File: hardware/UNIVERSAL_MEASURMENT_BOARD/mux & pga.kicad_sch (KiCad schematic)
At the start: 11 parts, among them U3 PGA280AIPW, U4 CD4097BM

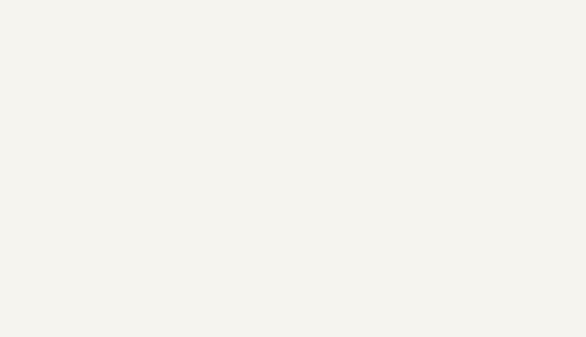
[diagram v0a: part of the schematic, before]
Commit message: clean up project visuals
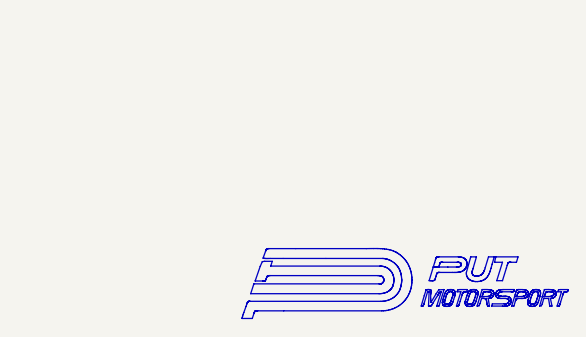
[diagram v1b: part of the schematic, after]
